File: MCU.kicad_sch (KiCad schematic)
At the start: 0 parts

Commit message: Add files via upload
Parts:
- added C10, C11, C12, C13: 100u, symbol Device:C
- added C14: 10u, symbol Device:C
- added C15: 10n, symbol Device:C
- added C16, C17: 1u, symbol Device:C
- added C18, C19: 10p, symbol Device:C
- added L3: 10n, symbol Device:L
- added R7: 10k, symbol Device:R_US
- added R8: 0R, symbol Device:R_US
- added U4: STM32F103CBTx, Package_QFP:LQFP-48_7x7mm_P0.5mm, symbol MCU_ST_STM32F1:STM32F103CBTx
- added Y1: 16Mhz, symbol Device:Crystal_GND24
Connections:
- new net +3V3: C10.1, C11.1, C12.1, C13.1, C14.1, C17.1, L3.2, U4.1 (VBAT), U4.24 (VDD), U4.36 (VDD), U4.48 (VDD)
- new net BOOT0: R7.2, U4.44 (BOOT0)
- new net GND: C10.2, C11.2, C12.2, C13.2, C14.2, C15.2, C16.2, C17.2, C18.2, C19.2, R7.1, U4.23 (VSS), U4.35 (VSS), U4.47 (VSS), U4.8 (VSSA), Y1.2, Y1.4
- new net HSE_IN: C18.1, U4.5 (PD0), Y1.1
- new net HSE_OUT: R8.2, U4.6 (PD1)
- new net NRST: U4.7 (NRST)
- new net VDDA: C15.1, C16.1, L3.1, U4.9 (VDDA)
- new net XTAL_IN: C19.1, R8.1, Y1.3
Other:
- note added: "CL = 10pF ESR = 80R"
- note added: "Crystal: AN2867"

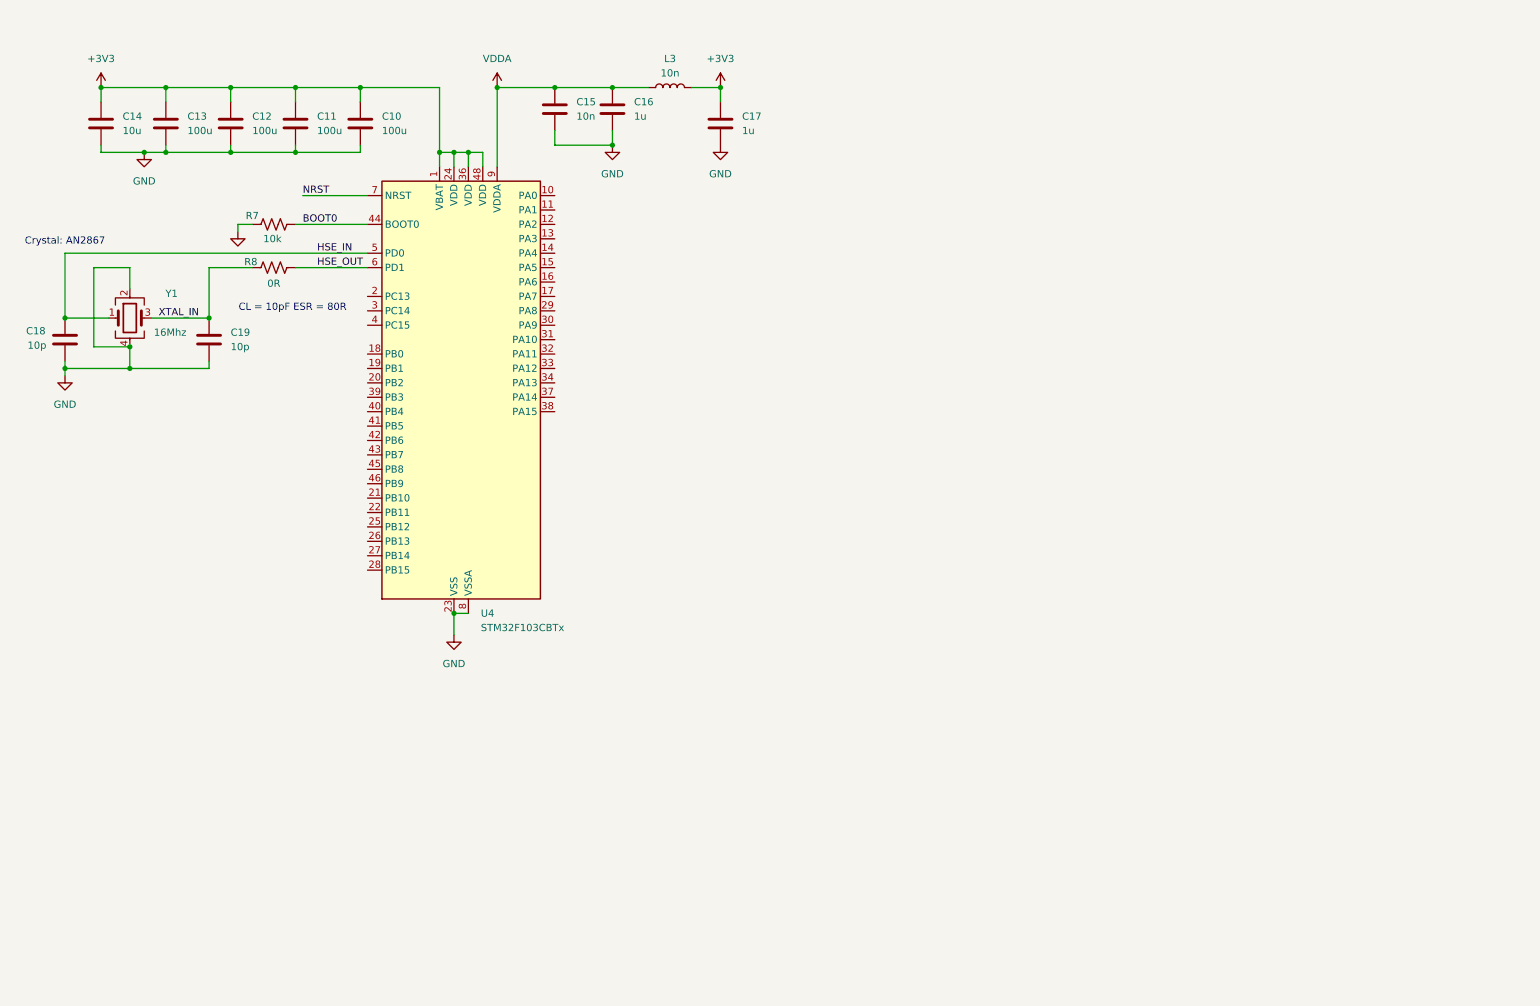
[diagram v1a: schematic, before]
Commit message: Adding official files from course download
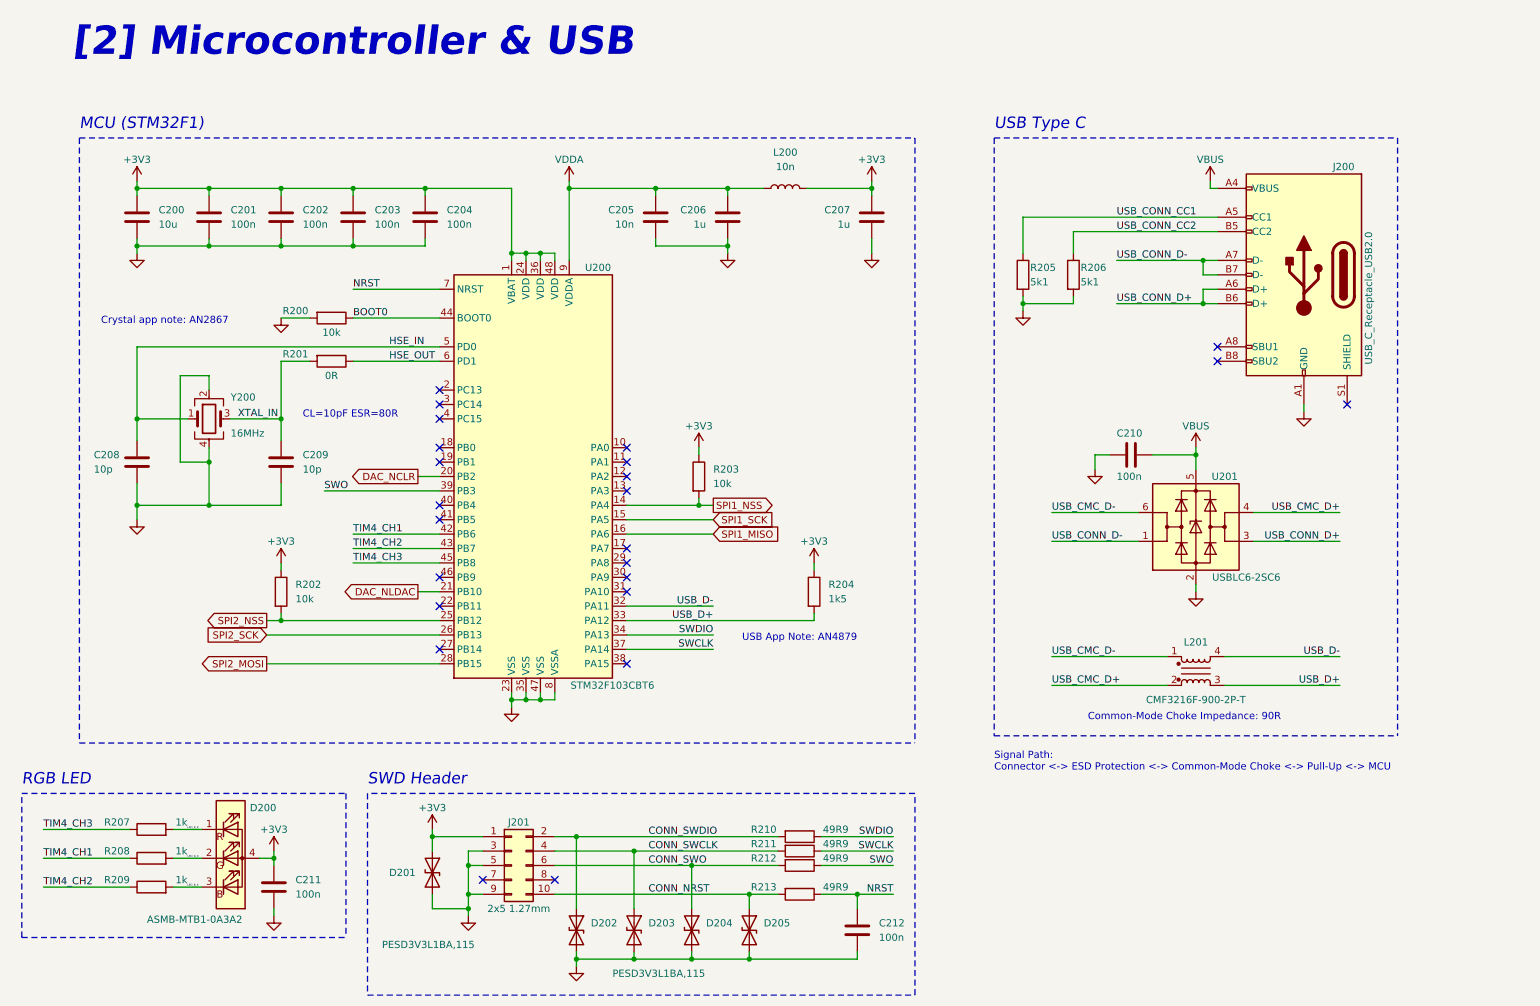
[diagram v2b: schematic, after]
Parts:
- removed C10, C11, C12, C13: 100u, symbol Device:C
- removed C14: 10u, symbol Device:C
- removed C15: 10n, symbol Device:C
- removed C16, C17: 1u, symbol Device:C
- removed C18, C19: 10p, symbol Device:C
- removed L3: 10n, symbol Device:L
- removed R7: 10k, symbol Device:R_US
- removed R8: 0R, symbol Device:R_US
- removed U4: STM32F103CBTx, Package_QFP:LQFP-48_7x7mm_P0.5mm, symbol MCU_ST_STM32F1:STM32F103CBTx
- removed Y1: 16Mhz, symbol Device:Crystal_GND24
- added C200: 10u, Capacitor_SMD:C_0603_1608Metric, symbol Device:C
- added C201, C202, C203, C204, C210, C211, C212: 100n, Capacitor_SMD:C_0402_1005Metric, symbol Device:C
- added C205: 10n, Capacitor_SMD:C_0402_1005Metric, symbol Device:C
- added C206, C207: 1u, Capacitor_SMD:C_0603_1608Metric, symbol Device:C
- added C208, C209: 10p, Capacitor_SMD:C_0402_1005Metric, symbol Device:C
- added D200: ASMB-MTB1-0A3A2, LED_SMD:LED_Avago_PLCC4_3.2x2.8mm_CW, symbol LED:ASMB-MTB1-0A3A2
- added D201, D202, D203, D204, D205: PESD3V3L1BA,115, Diode_SMD:D_SOD-323, symbol Device:D_TVS
- added J200: USB_C_Receptacle_USB2.0, Connector_USB:USB_C_Receptacle_HRO_TYPE-C-31-M-12, symbol Connector:USB_C_Receptacle_USB2.0
- added J201: 2x5 1.27mm, Connector_PinHeader_1.27mm:PinHeader_2x05_P1.27mm_Vertical_SMD, symbol Connector_Generic:Conn_02x05_Odd_Even
- added L200: 10n, Inductor_SMD:L_0402_1005Metric, symbol Device:L
- added L201: CMF3216F-900-2P-T, PhilsLab_Footprints_KiCad6:CMC-1206, symbol Device:EMI_Filter_LL_1423
- added R200, R202, R203: 10k, Resistor_SMD:R_0402_1005Metric, symbol Device:R
- added R201: 0R, Resistor_SMD:R_0402_1005Metric, symbol Device:R
- added R204: 1k5, Resistor_SMD:R_0402_1005Metric, symbol Device:R
- added R205, R206: 5k1, Resistor_SMD:R_0402_1005Metric, symbol Device:R
- added R207, R208, R209: 1k, Resistor_SMD:R_0402_1005Metric, symbol Device:R
- added R210, R211, R212, R213: 49R9, Resistor_SMD:R_0402_1005Metric, symbol Device:R
- added U200: STM32F103CBT6, Package_QFP:LQFP-48_7x7mm_P0.5mm, symbol MCU_ST_STM32F1:STM32F103CBTx
- added U201: USBLC6-2SC6, Package_TO_SOT_SMD:SOT-23-6, symbol Power_Protection:USBLC6-2SC6
- added Y200: 16MHz, Crystal:Crystal_SMD_3225-4Pin_3.2x2.5mm, symbol Device:Crystal_GND24
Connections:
- net +3V3: now also C200.1, C201.1, C202.1, C203.1, C204.1, C207.1, C211.1, D200.4 (A), D201.1 (A1), J201.1 (Pin_1), L200.2, R202.1, R203.1, R204.1, U200.1 (VBAT), U200.24 (VDD), U200.36 (VDD), U200.48 (VDD)
- net BOOT0: now also R200.1, U200.44 (BOOT0)
- net GND: now also C200.2, C201.2, C202.2, C203.2, C204.2, C205.2, C206.2, C207.2, C208.2, C209.2, C210.2, C211.2, C212.2, D201.2 (A2), D202.2 (A2), D203.2 (A2), D204.2 (A2), D205.2 (A2), J200.A1 (GND), J200.A12 (GND), J200.B1 (GND), J200.B12 (GND), J201.3 (Pin_3), J201.5 (Pin_5), J201.9 (Pin_9), R200.2, R205.2, R206.2, U200.23 (VSS), U200.35 (VSS), U200.47 (VSS), U200.8 (VSSA), U201.2 (GND), Y200.2, Y200.4
- net HSE_IN: now also C208.1, U200.5 (PD0), Y200.1
- net HSE_OUT: now also R201.1, U200.6 (PD1)
- net NRST: now also C212.1, R213.1, U200.7 (NRST)
- net VDDA: now also C205.1, C206.1, L200.1, U200.9 (VDDA)
- net XTAL_IN: now also C209.1, R201.2, Y200.3
- new net CONN_NRST: D205.1 (A1), J201.10 (Pin_10), R213.2
- new net CONN_SWCLK: D203.1 (A1), J201.4 (Pin_4), R211.2
- new net CONN_SWDIO: D202.1 (A1), J201.2 (Pin_2), R210.2
- new net CONN_SWO: D204.1 (A1), J201.6 (Pin_6), R212.2
- new net DAC_NCLR: U200.20 (PB2)
- new net DAC_NLDAC: U200.21 (PB10)
- new net LED_B_K: D200.3 (BK), R209.2
- new net LED_G_K: D200.2 (GK), R208.2
- new net LED_R_K: D200.1 (RK), R207.2
- new net SPI1_MISO: U200.16 (PA6)
- new net SPI1_NSS: R203.2, U200.14 (PA4)
- new net SPI1_SCK: U200.15 (PA5)
- new net SPI2_MOSI: U200.28 (PB15)
- new net SPI2_NSS: R202.2, U200.25 (PB12)
- new net SPI2_SCK: U200.26 (PB13)
- new net SWCLK: R211.1, U200.37 (PA14)
- new net SWDIO: R210.1, U200.34 (PA13)
- new net SWO: R212.1, U200.39 (PB3)
- new net TIM4_CH1: R208.1, U200.42 (PB6)
- new net TIM4_CH2: R209.1, U200.43 (PB7)
- new net TIM4_CH3: R207.1, U200.45 (PB8)
- new net USB_CMC_D+: L201.2, U201.4 (I/O2)
- new net USB_CMC_D-: L201.1, U201.6 (I/O1)
- new net USB_CONN_CC1: J200.A5 (CC1), R205.1
- new net USB_CONN_CC2: J200.B5 (CC2), R206.1
- new net USB_CONN_D+: J200.A6 (D+), J200.B6 (D+), U201.3 (I/O2)
- new net USB_CONN_D-: J200.A7 (D-), J200.B7 (D-), U201.1 (I/O1)
- new net USB_D+: L201.3, R204.2, U200.33 (PA12)
- new net USB_D-: L201.4, U200.32 (PA11)
- new net VBUS: C210.1, J200.A4 (VBUS), J200.A9 (VBUS), J200.B4 (VBUS), J200.B9 (VBUS), U201.5 (VBUS)
- no-connect marks 0 -> 24
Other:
- note added: "CL=10pF ESR=80R"
- note added: "Common-Mode Choke Impedance: 90R"
- note added: "Crystal app note: AN2867"
- note added: "MCU (STM32F1)"
- note added: "RGB LED"
- note added: "SWD Header"
- note added: "Signal Path: Connector <-> ESD Protection <-> Common-Mode Choke <-> Pull-Up <-> MCU"
- note added: "USB App Note: AN4879"
- note added: "USB Type C"
- note added: "[2] Microcontroller & USB"
- note removed: "CL = 10pF ESR = 80R"
- note removed: "Crystal: AN2867"
- company: (none) -> Phil's Lab
- title: (none) -> Mixed-Signal Demo PCB
